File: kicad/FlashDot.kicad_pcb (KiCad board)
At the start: 2 copper layers, 34.5 x 33.5 mm, 7 parts, among them Q2 Q_NPN_EBC

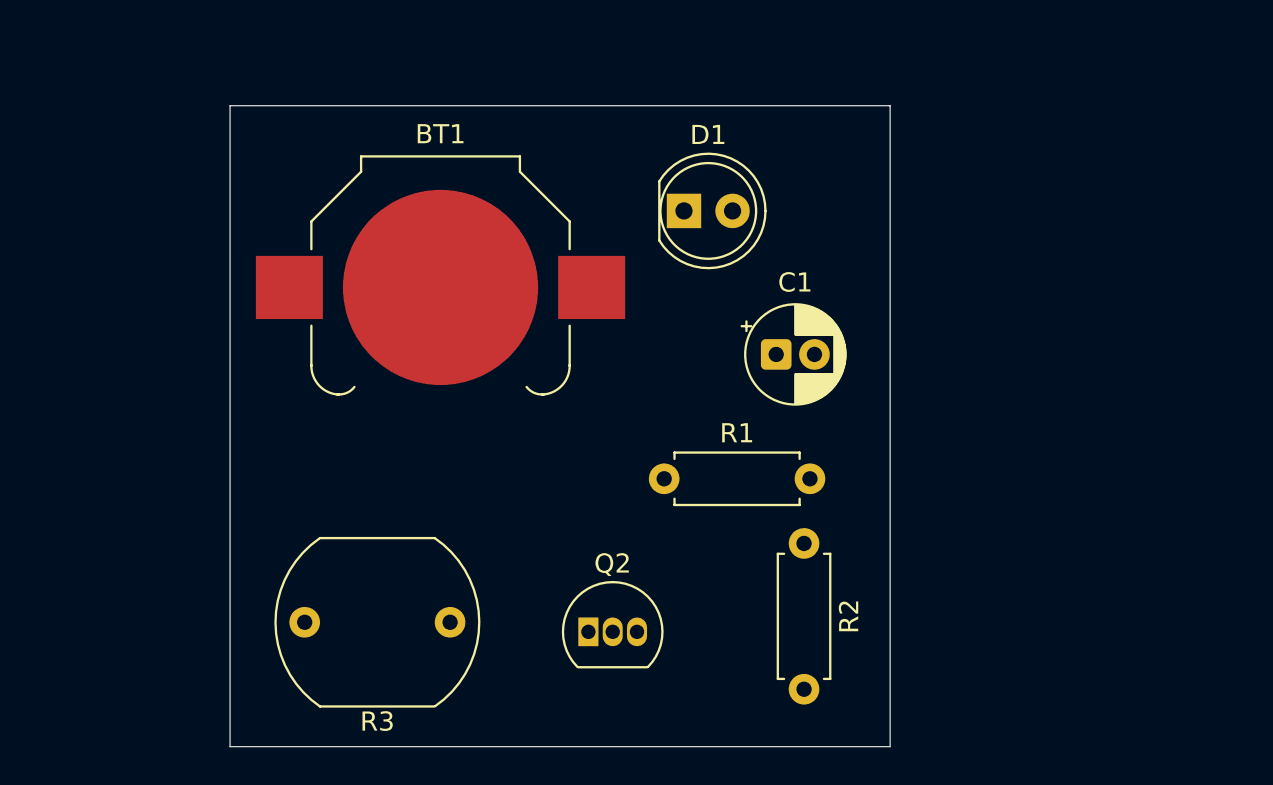
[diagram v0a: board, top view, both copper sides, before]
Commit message: Done
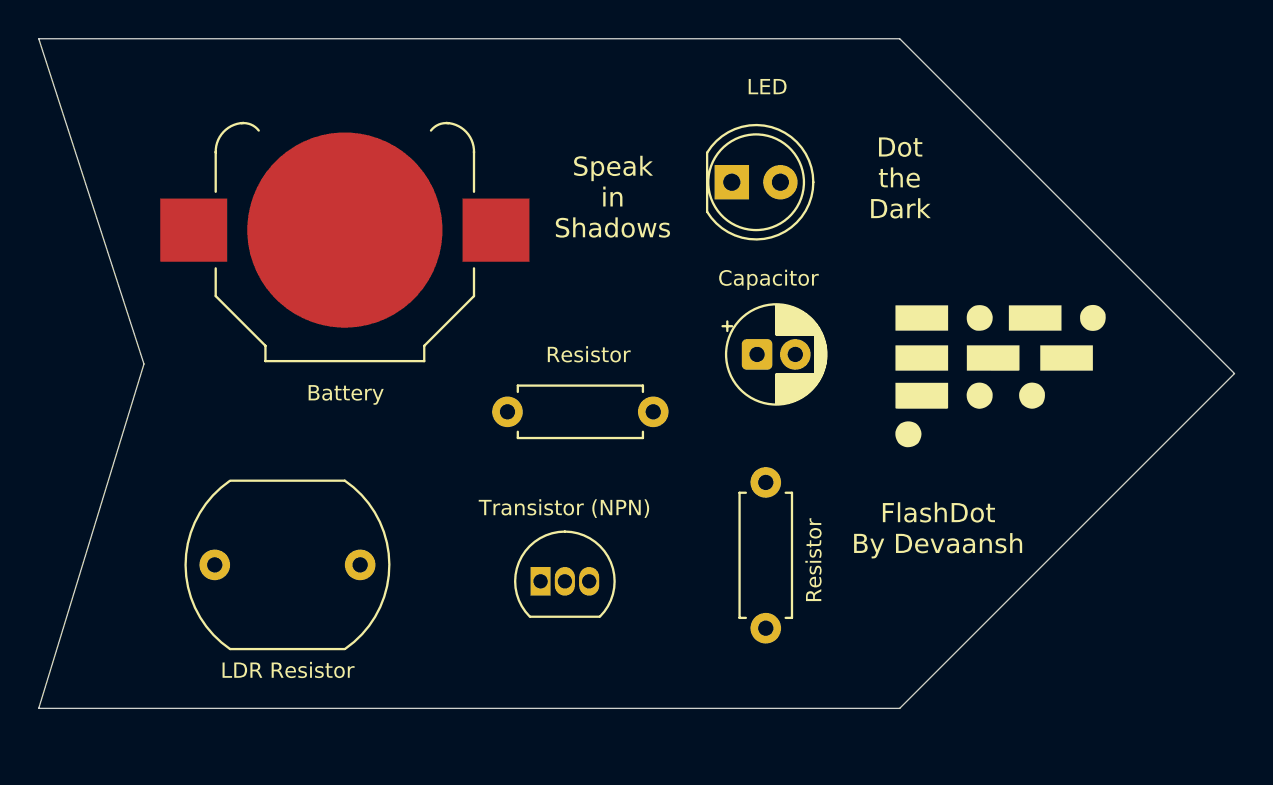
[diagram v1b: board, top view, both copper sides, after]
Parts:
- moved R1 8.91 mm to (124.5, 79.5)
- moved BT1 5.83 mm to (116.0, 70.0), turned to 180 degrees
- moved R3 5.58 mm to (116.8, 87.5)
- moved R2 3.77 mm to (138.0, 83.2)
- moved Q2 3.64 mm to (126.2, 88.4)
- moved D1 2.92 mm to (136.2, 67.5)
- moved C1 1.00 mm to (137.5, 76.5)
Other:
- board size 34.5 x 33.5 mm -> 62.5 x 35 mm
- board text added: "Battery"
- board text added: "Capacitor"
- board text added: "Dot the Dark"
- board text added: "FlashDot By Devaansh"
- board text added: "LDR Resistor"
- board text added: "LED"
- board text added: "Resistor"
- board text added: "Speak in Shadows"
- board text added: "Transistor (NPN)"
